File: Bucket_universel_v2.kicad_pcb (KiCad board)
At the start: 2 copper layers, 100 x 60.5 mm, 128 parts, among them J1 Conn_02x11_Odd_Even, J10 Conn_01x03, J11 Conn_01x03, J12 Conn_01x04_Pin, J13 SM03B-SRSS-TB, J14 Conn_02x18_Odd_Even, J15 USB_C_Receptacle_USB2.0_16P, J2 Conn_01x03_Pin, J3 Conn_01x05_Pin, J4 Conn_01x04_Pin, J5 Conn_01x04_Pin, J7 Conn_02x18_Odd_Even, J8 Conn_01x03, J9 Conn_01x02_Pin, SW1 SW_Push, SW2 SW_Push, U1 DRV8825PWPR, U10 SN74LVC1T45DBV, U11 DRV8874PWPR, U12 LM7805MP/NOPB, U2 DRV8874PWPR, U3 W25Q128JVS, U4 NCP1117-3.3_SOT223, U5 RP2350_60QFN, U7 SN74LVC1T45DBV, U8 AOZ2261AQI-15, U9 SN74LVC1T45DBV, Y1 ABM8-272-T3

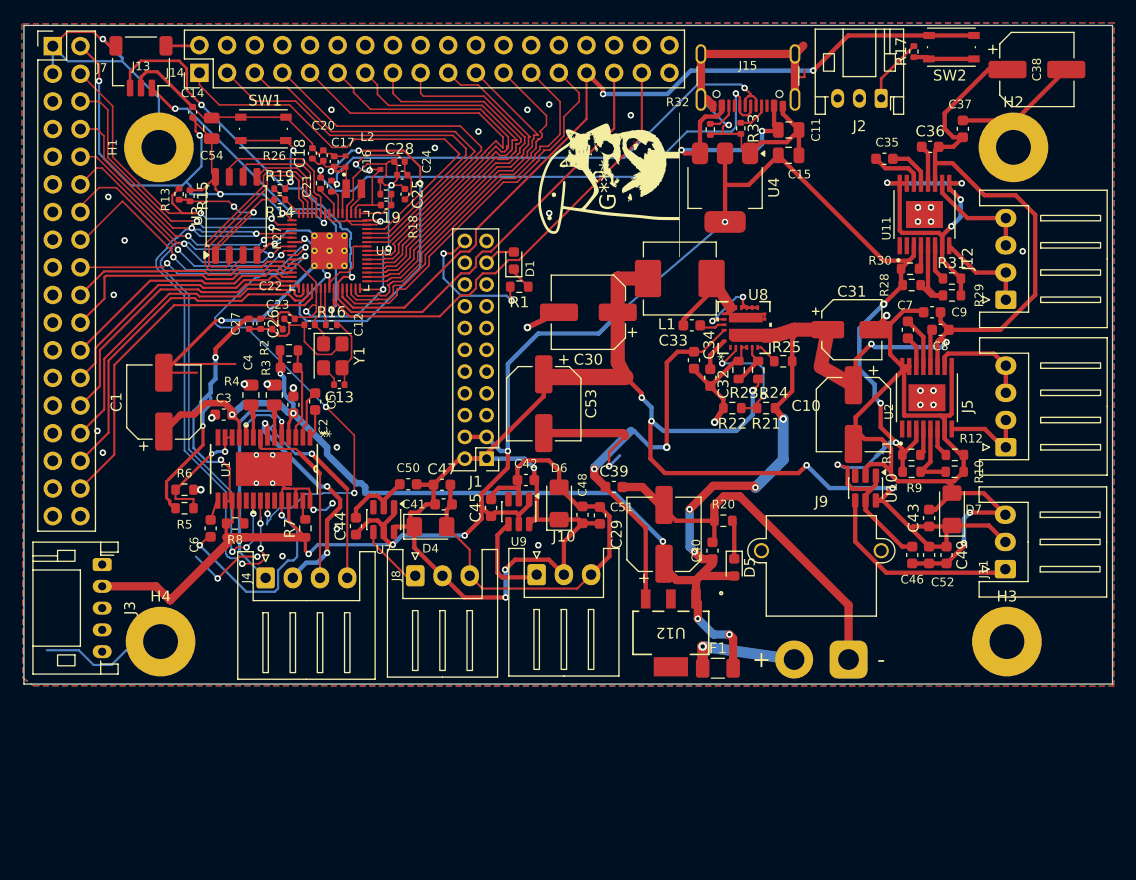
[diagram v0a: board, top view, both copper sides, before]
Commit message: V3
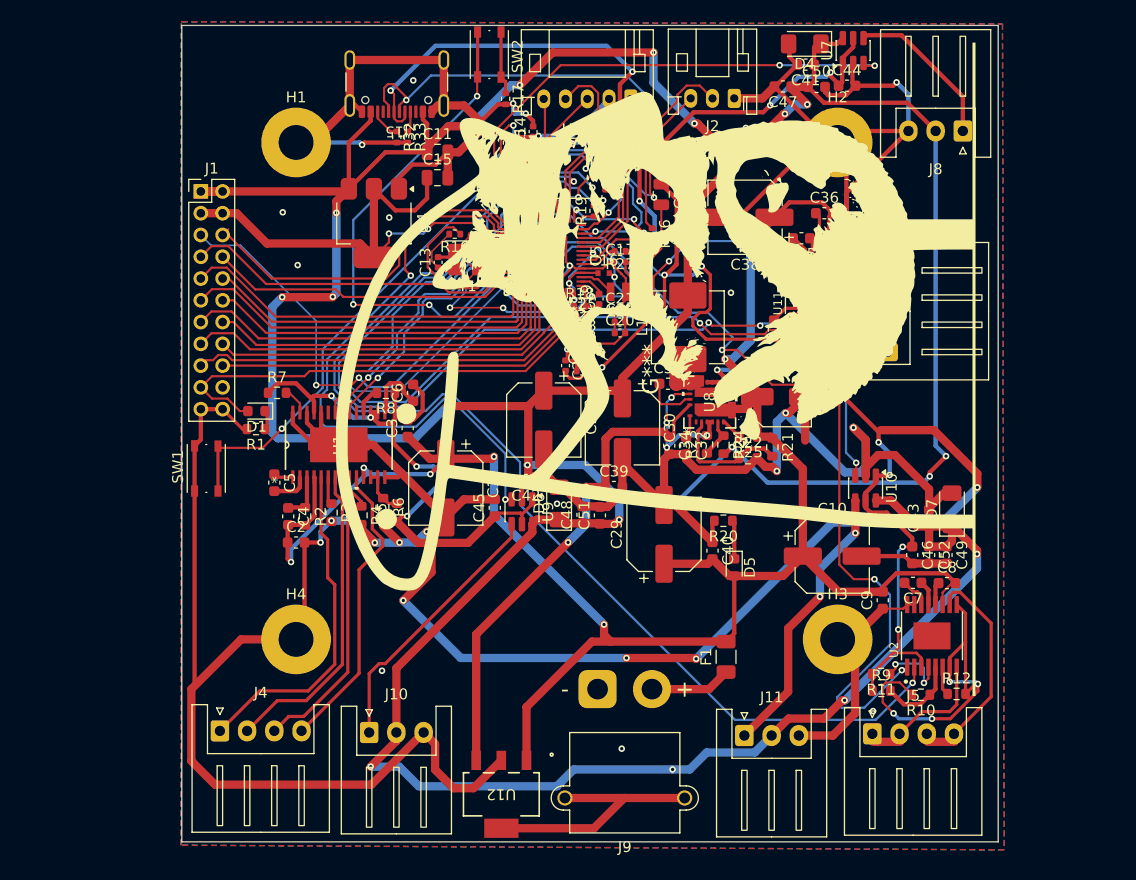
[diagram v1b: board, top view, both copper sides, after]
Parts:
- removed J13: SM03B-SRSS-TB, Connector_JST:JST_SH_SM03B-SRSS-TB_1x03-1MP_P1.00mm_Horizontal
- removed J14, J7: Conn_02x18_Odd_Even, Connector_PinHeader_2.54mm:PinHeader_2x18_P2.54mm_Vertical
- J15: footprint Rework_local:USB4105_GND_heel_relief -> Connector_USB:USB_C_Receptacle_GCT_USB4105-xx-A_16P_TopMnt_Horizontal
- R3, R4: value 220m 0.5W 1% -> 100m; footprint Resistor_SMD:R_0805_2012Metric -> Resistor_SMD:R_0603_1608Metric
- R5: value 20k -> 23k
- U1: footprint DRV8825_local:PWP28_TI_1p5x0p45_EP3p1x5p18 -> DRV8825:PWP28_5P18X3P1
- U11, U2: value DRV8874PWPR -> a
- U12: value LM7805MP/NOPB -> L7805
- U8: footprint AOZ2261AQI_15:QFN4X4-22L_EP2_S_AOS -> footprints:QFN4X4-22L_EP2_S_AOS
- moved J8 64.8 mm to (218.0, 66.4), turned to 180 degrees
- moved J3 64.7 mm to (187.5, 63.5), turned to 180 degrees
- moved U7 61.0 mm to (207.9, 59.1), turned to 90 degrees
- moved C44 60.6 mm to (207.4, 62.3), turned to 0 degrees
- moved D4 56.1 mm to (203.5, 58.4), turned to 180 degrees
- moved C50 52.3 mm to (204.6, 62.4), turned to 0 degrees
- moved C41 52.3 mm to (203.6, 60.4), turned to 180 degrees
- moved C47 48.2 mm to (201.5, 62.4), turned to 180 degrees
- moved SW2 42.5 mm to (174.5, 59.4), turned to -90 degrees
- moved C54 41.7 mm to (190.3, 72.3), turned to -90 degrees
- moved R17 37.8 mm to (176.0, 63.5), turned to -90 degrees
- moved J1 35.9 mm to (148.0, 72.0), turned to 0 degrees
- moved U4 32.4 mm to (163.9, 74.9)
- moved C11 32.3 mm to (169.7, 68.4)
- moved C15 32.3 mm to (169.7, 70.7)
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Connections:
- C11 pad 1: VBUS -> +5V
- J15 pad A4: VBUS -> +5V
- J15 pad A9: VBUS -> +5V
- J15 pad B4: VBUS -> +5V
- J15 pad B9: VBUS -> +5V
- R13 pad 1: /Microcontroller/GPIO0 -> GPIO0
- U11 pad 17: GND -> (no net)
- U12 pad 4: GND -> (no net)
- U2 pad 17: GND -> (no net)
- U4 pad 3: VBUS -> +5V
- U5 pad 12: /Microcontroller/GPIO8 -> GPIO8
- U5 pad 13: /Microcontroller/GPIO9 -> GPIO9
- U5 pad 14: /Microcontroller/GPIO10 -> GPIO10
- U5 pad 15: /Microcontroller/GPIO11 -> GPIO11
- U5 pad 16: /Microcontroller/GPIO12 -> GPIO12
- U5 pad 17: /Microcontroller/GPIO13 -> GPIO13
- U5 pad 18: /Microcontroller/GPIO14 -> GPIO14
- U5 pad 19: /Microcontroller/GPIO15 -> GPIO15
- U5 pad 2: /Microcontroller/GPIO0 -> GPIO0
- U5 pad 27: /Microcontroller/GPIO16 -> GPIO16
- U5 pad 28: /Microcontroller/GPIO17 -> GPIO17
- U5 pad 29: /Microcontroller/GPIO18 -> GPIO18
- U5 pad 3: /Microcontroller/GPIO1 -> GPIO1
- U5 pad 31: /Microcontroller/GPIO19 -> GPIO19
- U5 pad 32: /Microcontroller/GPIO20 -> GPIO20
- U5 pad 33: /Microcontroller/GPIO21 -> GPIO21
- U5 pad 34: /Microcontroller/GPIO22 -> GPIO22
- U5 pad 35: /Microcontroller/GPIO23 -> GPIO23
- U5 pad 36: /Microcontroller/GPIO24 -> GPIO24
- U5 pad 37: /Microcontroller/GPIO25 -> GPIO25
- U5 pad 40: /Microcontroller/GPIO26_ADC0 -> GPIO26
- U5 pad 41: /Microcontroller/GPIO27_ADC1 -> GPIO27
- U5 pad 42: /Microcontroller/GPIO28_ADC2 -> GPIO28
- U5 pad 43: /Microcontroller/GPIO29_ADC3 -> GPIO29
- U5 pad 5: /Microcontroller/GPIO3 -> GPIO3
- U5 pad 8: /Microcontroller/GPIO5 -> GPIO5
- U5 pad 9: /Microcontroller/GPIO6 -> GPIO6
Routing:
- net +5V: track 157.6 -> 400.4 mm, vias 8 -> 19
- net GND: track 486.9 -> 600.7 mm, vias 60 -> 43
- net GPIO9: track 0.00 -> 100.4 mm, vias 0 -> 2
- net GPIO8: track 0.00 -> 80.4 mm, vias 0 -> 4
- net /Microcontroller/SWD: track 75.8 -> 0.00 mm, vias 2 -> 0
- net /Microcontroller/SWCLK: track 74.4 -> 0.00 mm, vias 2 -> 0
- net GPIO11: track 0.00 -> 72.2 mm, vias 0 -> 2
- net GPIO10: track 0.00 -> 71.8 mm, vias 0 -> 4
- net GPIO16: track 0.00 -> 58.7 mm, vias 0 -> 4
- net GPIO14: track 0.00 -> 56.4 mm, vias 0 -> 2
- net /Microcontroller/~{USB_BOOT}: track 9.15 -> 63.0 mm, vias 2 -> 4
- net GPIO15: track 0.00 -> 49.1 mm, vias 0 -> 3
- net GPIO12: track 0.00 -> 47.7 mm, vias 0 -> 2
- net +3V3: track 338.5 -> 385.3 mm, vias 22 -> 32
- net GPIO2: track 76.0 -> 31.8 mm, vias 5 -> 2
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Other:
- board size 100 x 60.5 mm -> 75 x 75 mm
